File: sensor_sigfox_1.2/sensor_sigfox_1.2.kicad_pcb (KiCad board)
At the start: 2 copper layers, 27.3 x 60.1 mm, 15 parts, among them IC1 WSSFM11R2DAT, J1 Battery, J2 Conn_01x07_Socket, U1 ATtiny826-X, U2 MLX90393, Y1 32.768 kHz

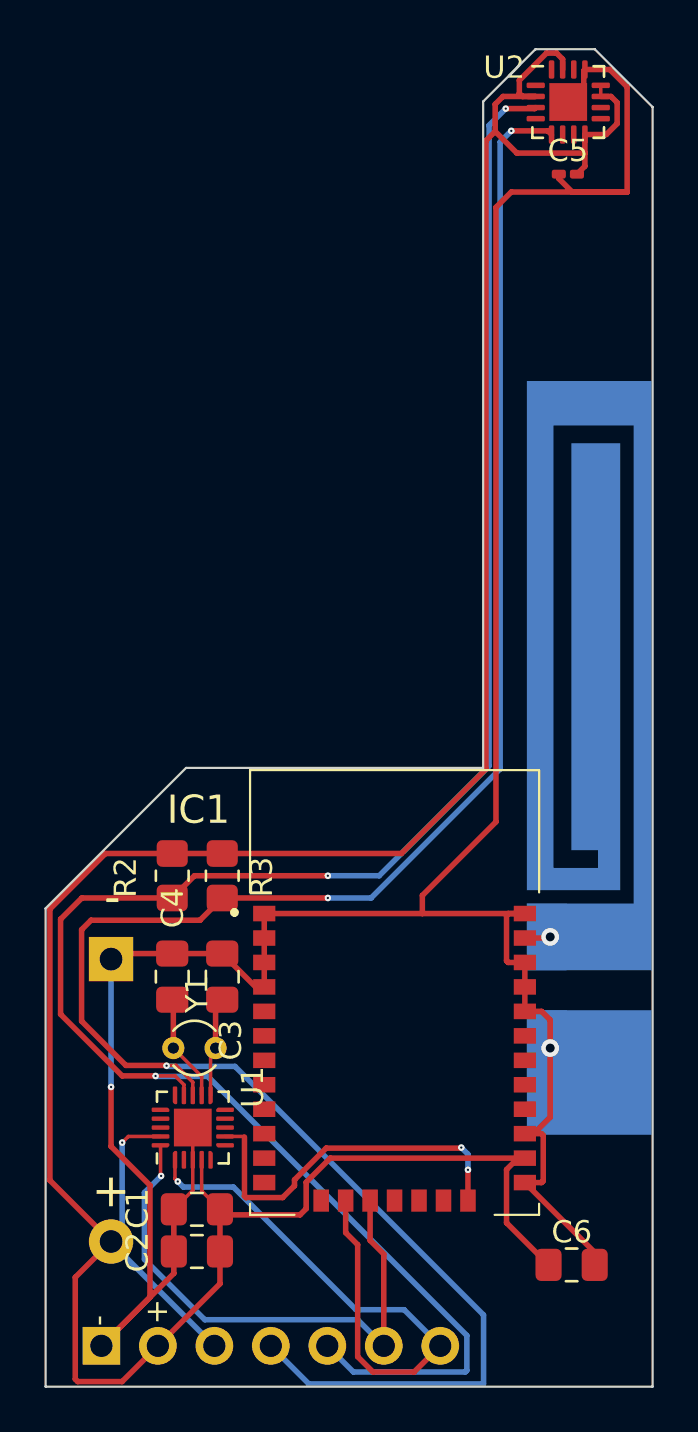
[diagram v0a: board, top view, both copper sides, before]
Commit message: gerber y conexiones int/trig
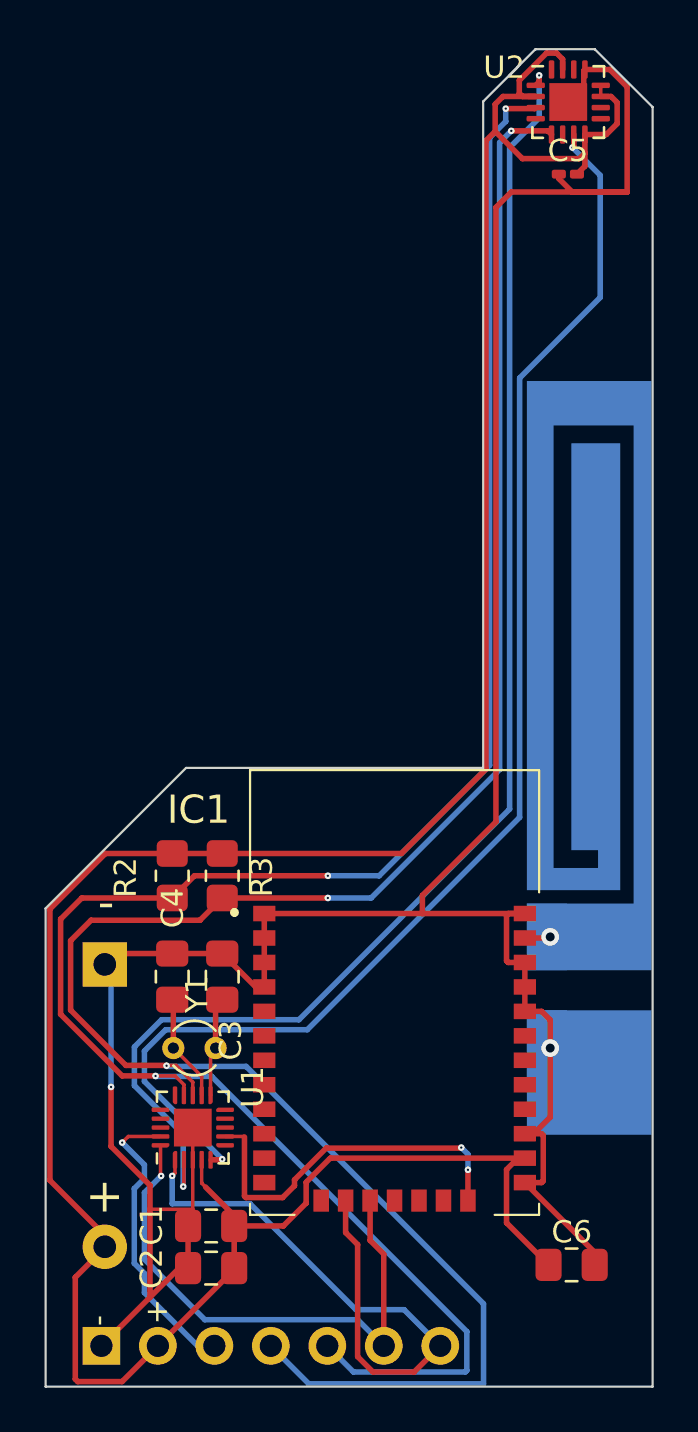
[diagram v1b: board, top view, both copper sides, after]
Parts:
- moved C1 0.99 mm to (121.2, 88.9)
- moved C2 0.99 mm to (121.2, 90.8)
- moved J1 0.37 mm to (116.4, 77.1)
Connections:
- U1 pad 2: unconnected-(U1-PA3-Pad2) -> Net-(U1-PA3)
- U1 pad 5: unconnected-(U1-PA4-Pad5) -> Net-(U1-PA4)
- U2 pad 1: unconnected-(U2-INT-Pad1) -> Net-(U1-PA3)
- U2 pad 7: unconnected-(U2-INT/TRIG-Pad7) -> Net-(U1-PA4)
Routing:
- net Net-(U1-PA3): track 0.00 -> 63.8 mm, vias 0 -> 2
- net Net-(U1-PA4): track 0.00 -> 60.8 mm, vias 0 -> 2
- net GND: track 132.6 -> 130.8 mm
- net /SF_TX: track 27.6 -> 28.5 mm
- net Net-(J2-Pin_3): track 12.7 -> 13.5 mm
- net /SDA: track 95.7 -> 96.4 mm
